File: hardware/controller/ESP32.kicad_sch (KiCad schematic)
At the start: 35 parts, among them J1 Conn_01x05_Pin, Q1 SS8050-G, Q2 SS8050-G, U1 ESP32-S3, Y1 FH4000074Z

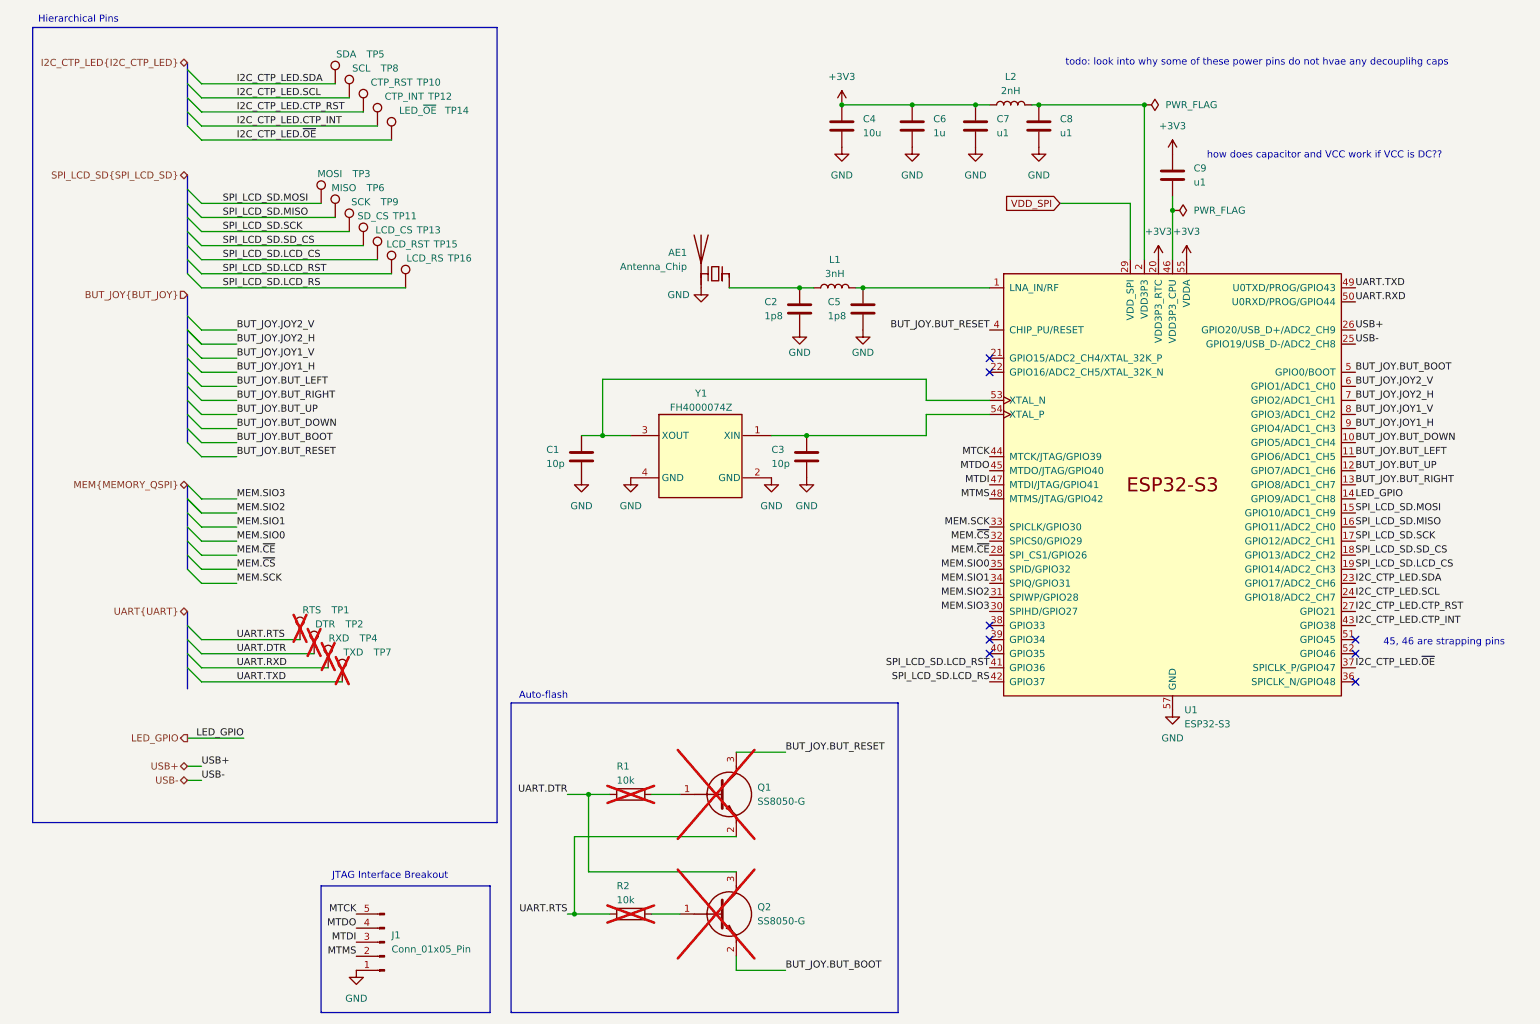
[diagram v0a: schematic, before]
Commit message: forgor
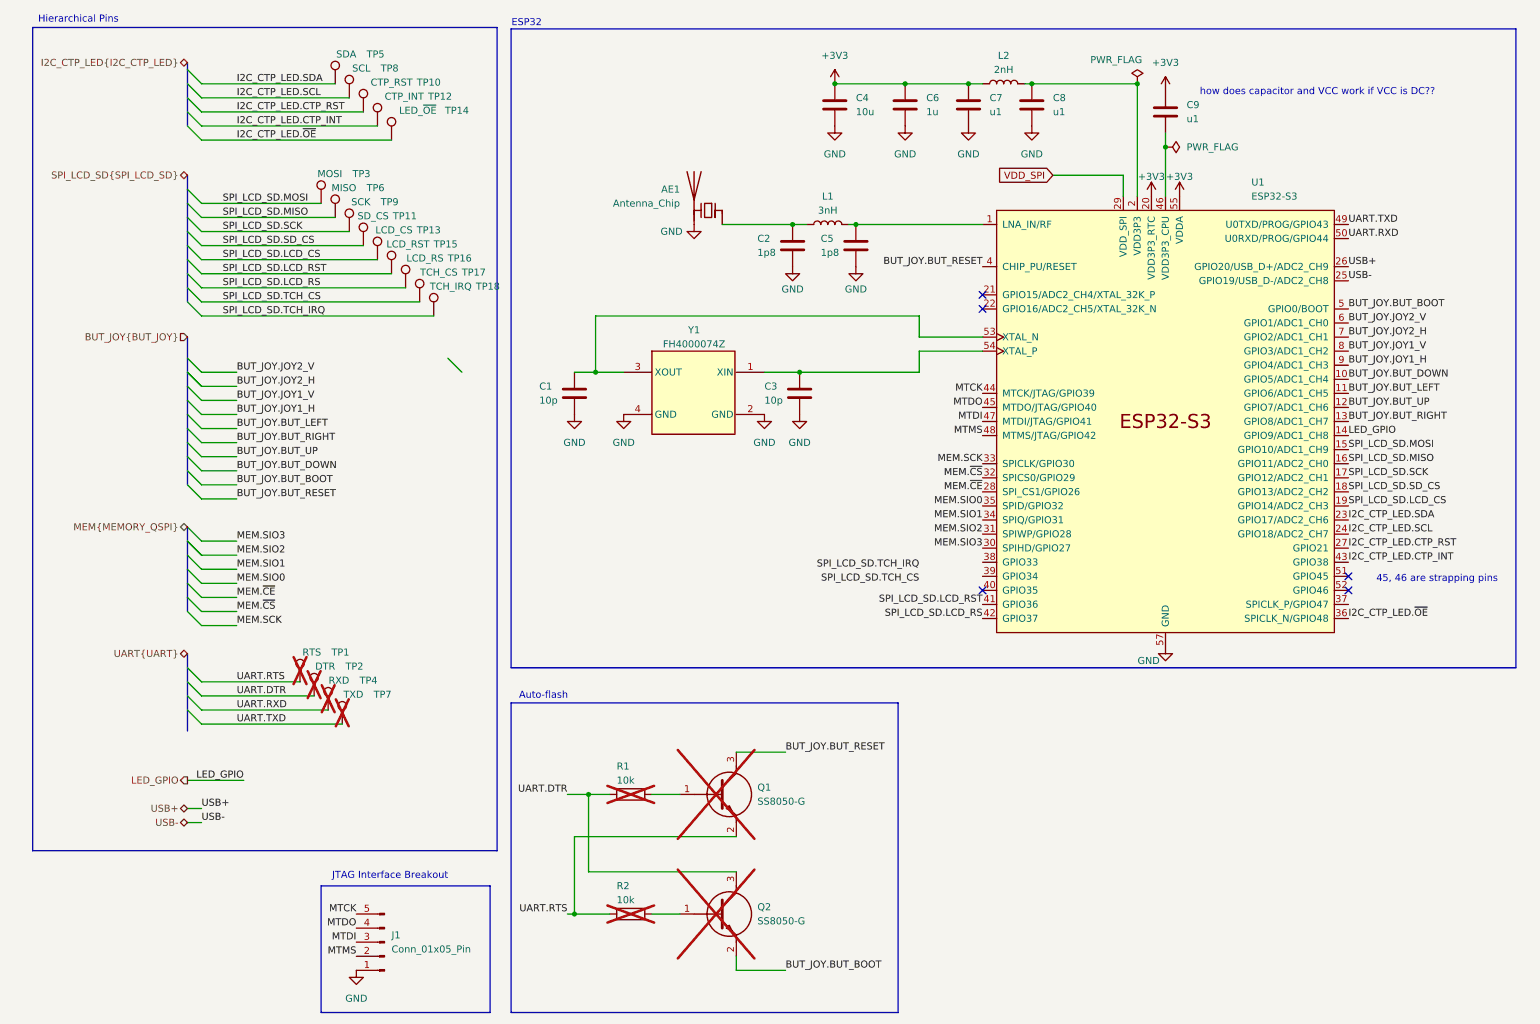
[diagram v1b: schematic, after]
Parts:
- added TP17: TCH_CS, SamacSys_Parts:5000, symbol Connector:TestPoint
- added TP18: TCH_IRQ, SamacSys_Parts:5000, symbol Connector:TestPoint
- TP10, TP11, TP12, TP13, TP14, TP15, TP16, TP3, TP5, TP6, TP8, TP9: footprint 5000 -> SamacSys_Parts:5000
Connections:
- net I2C_CTP_LED.~{OE}: now also U1.36 (SPICLK_N/GPIO48); no longer U1.37 (SPICLK_P/GPIO47)
- new net SPI_LCD_SD.TCH_CS: TP17.1
- new net SPI_LCD_SD.TCH_IRQ: TP18.1
- no-connect marks 8 -> 5
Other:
- note added: "ESP32"
- note removed: "todo: look into why some of these power pins do not hvae any decouplihg caps"
- moved on the sheet: AE1, C1, C2, C3, C4, C5, C6, C7, C8, C9, L1, L2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
